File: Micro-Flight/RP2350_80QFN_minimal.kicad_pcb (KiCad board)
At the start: 4 copper layers, 48.5 x 62.5 mm, 61 parts, among them J5 USB_C_Receptacle_USB2.0_14P, U1 RP2350_80QFN, U2 E22-900M30S, U3 W25Q128JVS, U5 LC86G, U6 NCP1117-3.3_SOT223, Y1 ABM8-272-T3

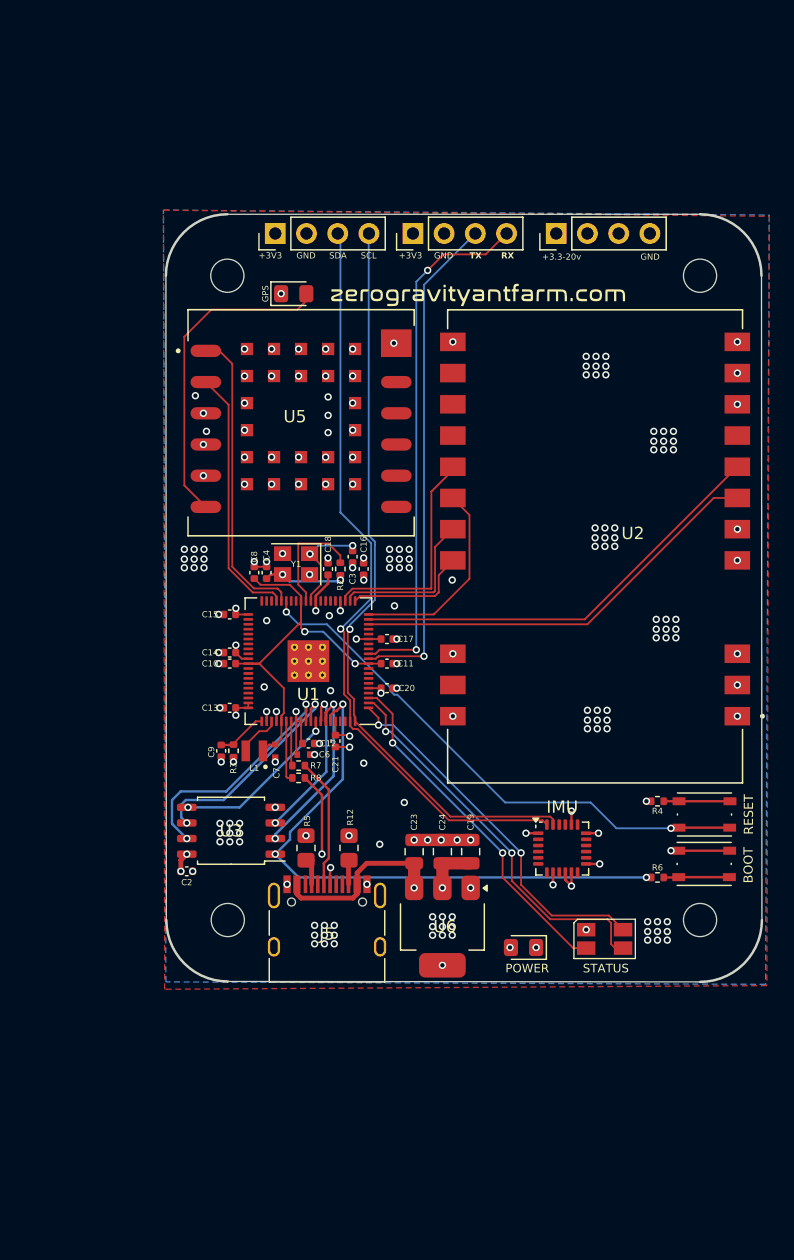
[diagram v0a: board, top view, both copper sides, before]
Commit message: REV B
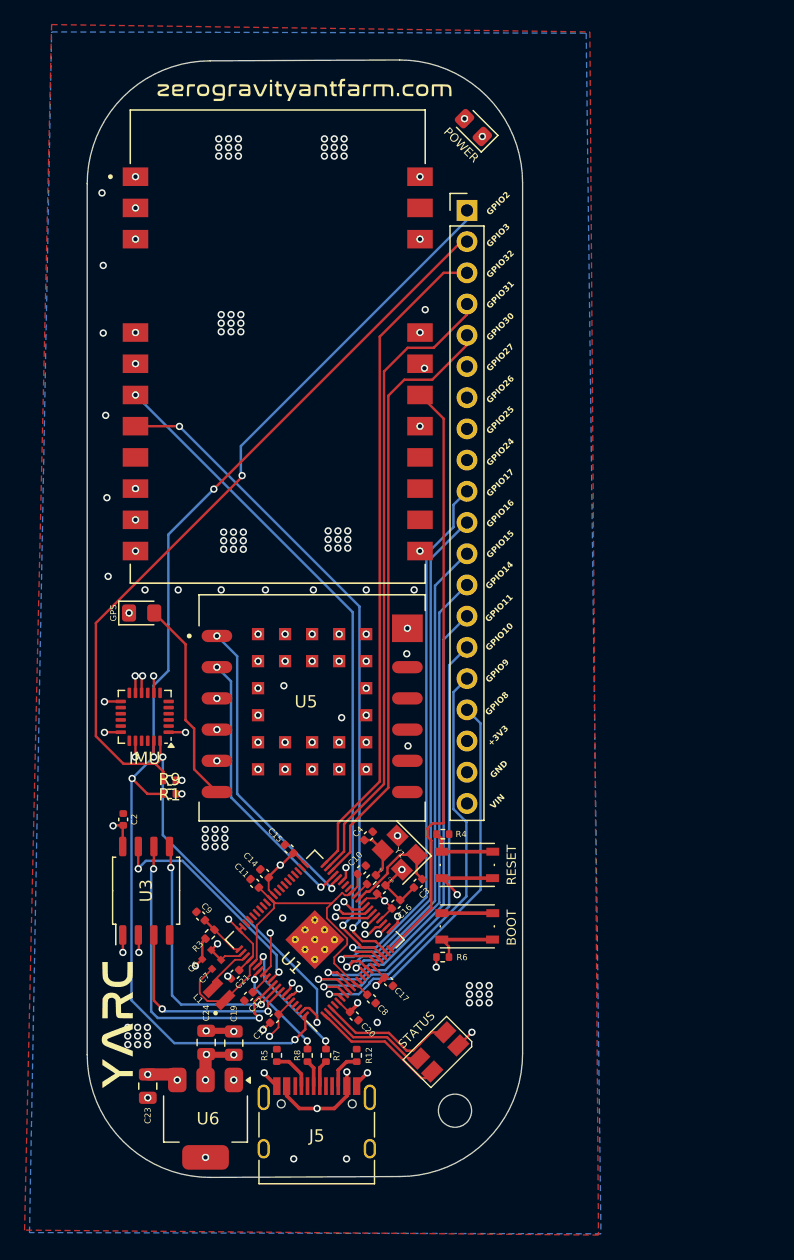
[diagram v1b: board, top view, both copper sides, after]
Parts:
- removed +3.3-20v, I2C, UART: Conn_01x04_Pin, Connector_PinHeader_2.54mm:PinHeader_1x04_P2.54mm_Vertical
- removed the G*** at (175.0, 99.7)
- removed the G*** at (141.9, 119.7)
- removed the G*** at (157.8, 102.6)
- removed the G*** at (162.0, 74.1)
- removed the G*** at (147.5, 103.6)
- removed the G*** at (168.4, 84.9)
- removed the G*** at (175.1, 79.3)
- removed the G*** at (139.9, 104.0)
- removed the G*** at (143.5, 131.9)
- removed the G*** at (154.9, 123.2)
- removed H1, H2, H4: MountingHole, MountingHole:MountingHole_2.7mm_M2.5
- added G***: LOGO, LOGO, F.Cu at (129.7, 136.0)
- added G***: LOGO, LOGO, B.Cu at (142.8, 116.3)
- added G***: LOGO, LOGO, B.Cu at (156.5, 35.5)
- added J2: Conn_01x20, Connector_PinHeader_2.54mm:PinHeader_1x20_P2.54mm_Vertical, F.Cu at (158.0, 70.2)
- added R1: 4.7k, Resistor_SMD:R_0402_1005Metric, F.Cu at (133.8, 116.6)
- added R9: 4.7k, Resistor_SMD:R_0402_1005Metric, F.Cu at (133.8, 117.7)
- R12, R5: footprint Resistor_SMD:R_0805_2012Metric_Pad1.20x1.40mm_HandSolder -> Resistor_SMD:R_0402_1005Metric
- moved H3 70.8 mm to (157.0, 143.5)
- moved POWER 66.8 mm to (158.5, 63.5), turned to 135 degrees
- moved C8 36.0 mm to (150.2, 134.4), turned to -45 degrees
- moved IMU 35.6 mm to (131.8, 111.4), turned to 180 degrees
- moved U2 30.5 mm to (142.6, 81.3), turned to 180 degrees
- moved C23 28.9 mm to (132.0, 141.5), turned to -90 degrees
- moved GPS 28.8 mm to (131.5, 103.0)
- moved C17 27.9 mm to (151.6, 133.0), turned to -45 degrees
- moved C16 27.4 mm to (152.2, 126.7), turned to 45 degrees
- moved C3 27.1 mm to (154.0, 125.0), turned to -135 degrees
- moved C20 26.8 mm to (148.8, 135.8), turned to -45 degrees
- moved C18 26.4 mm to (151.0, 125.5), turned to 45 degrees
- moved C13 25.5 mm to (142.3, 136.0), turned to -135 degrees
- moved R2 25.4 mm to (150.2, 124.7), turned to 45 degrees
- moved Y1 24.9 mm to (152.5, 122.5), turned to 135 degrees
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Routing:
- net /GPIO25: track 0.00 -> 69.0 mm, vias 0 -> 1
- net /GPIO26: track 0.00 -> 59.5 mm, vias 0 -> 1
- net /GPIO32: track 0.00 -> 54.0 mm
- net /GPIO31: track 0.00 -> 51.8 mm
- net /GPIO27: track 0.00 -> 50.2 mm, vias 0 -> 1
- net /GPIO30: track 0.00 -> 49.5 mm
- net /GPIO17: track 0.00 -> 44.8 mm, vias 0 -> 1
- net /GPIO21: track 10.2 -> 54.6 mm, vias 0 -> 2
- net /GPIO16: track 0.00 -> 44.4 mm, vias 0 -> 1
- net /GPIO13: track 42.9 -> 0.00 mm, vias 2 -> 0
- net /GPIO24: track 0.00 -> 42.5 mm, vias 0 -> 1
- net /GPIO15: track 0.00 -> 41.1 mm, vias 0 -> 1
- net /GPIO12: track 40.7 -> 0.00 mm, vias 1 -> 0
- net /GPIO22: track 13.1 -> 53.2 mm, vias 0 -> 2
- net /GPIO11: track 0.00 -> 38.6 mm, vias 0 -> 1
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- added copper zone on In2.Cu, net +3V3
- removed copper zone on In2.Cu, net GND
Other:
- board size 48.5 x 62.5 mm -> 35.4 x 90.9 mm
- board text added: "GPIO10"
- board text added: "GPIO11"
- board text added: "GPIO14"
- board text added: "GPIO15"
- board text added: "GPIO16"
- board text added: "GPIO17"
- board text added: "GPIO2"
- board text added: "GPIO24"
- board text added: "GPIO25"
- board text added: "GPIO26"
- board text added: "GPIO27"
- board text added: "GPIO3"
- board text added: "GPIO30"
- board text added: "GPIO31"
- board text added: "GPIO32"
- board text added: "GPIO8"
- board text added: "GPIO9"
- board text added: "VIN"
- board text removed: "RX"
- board text removed: "SCL"
- board text removed: "SDA"
- board text removed: "TX"
